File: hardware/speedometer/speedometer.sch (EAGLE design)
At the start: 129 parts, among them IC1 PIC32MX274F256DT-I_PT, IC10 TPS63001DRCT, IC11 TPS63002DRCT, IC12 SN65220DBVRG4, IC2 CSTCE8M00G55-R0, IC3 HM-11, IC4 BQ27441DRZR-G1A, IC5 BQ24075RGTT, IC6 NRF24L01P-T, IC7 CSTCE16M0V53-R0, IC8 24LC024ST, IC9 MAX16054AZT+T, J1 10104111-0001LF, J2 BAT, J3 CONUFL001-SMD-T, J4 Right_sens, J5 Right, J6 Left_sens, J7 Left, Q1 BC817, Q2 BC817, Q3 BC817, Q4 BC817, U1 SN74AHC1G08DBVR, U2 SN74AHC1G08DBVR, X1 TSW-102-07-G-S, X2 TSW-102-07-G-S

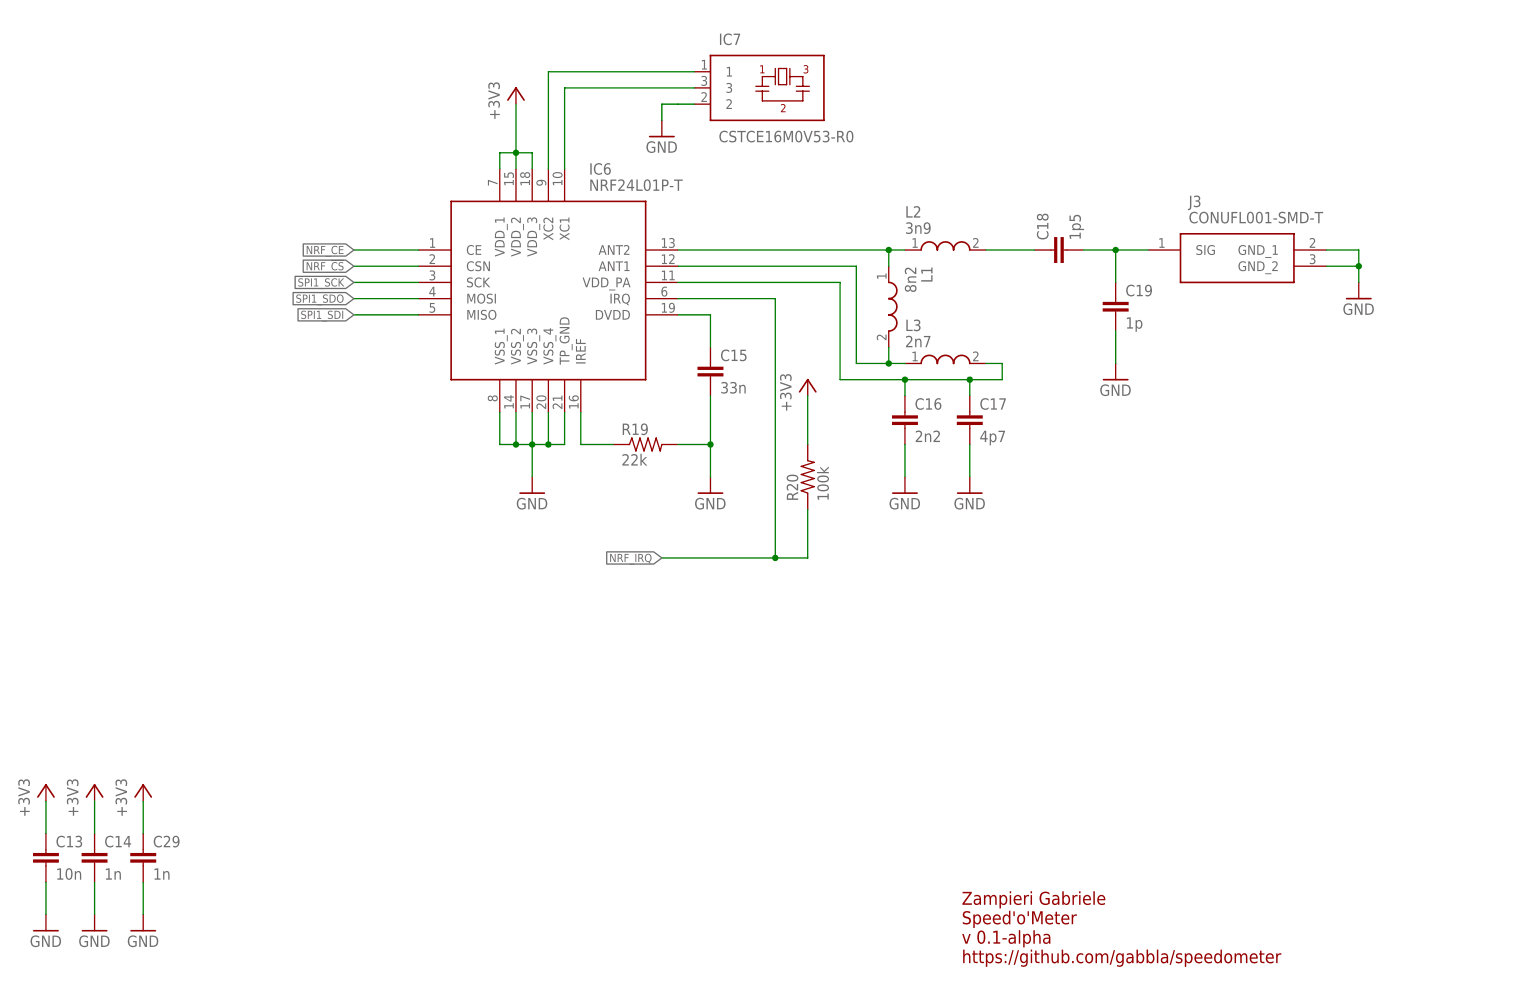
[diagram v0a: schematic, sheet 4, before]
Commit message: wip
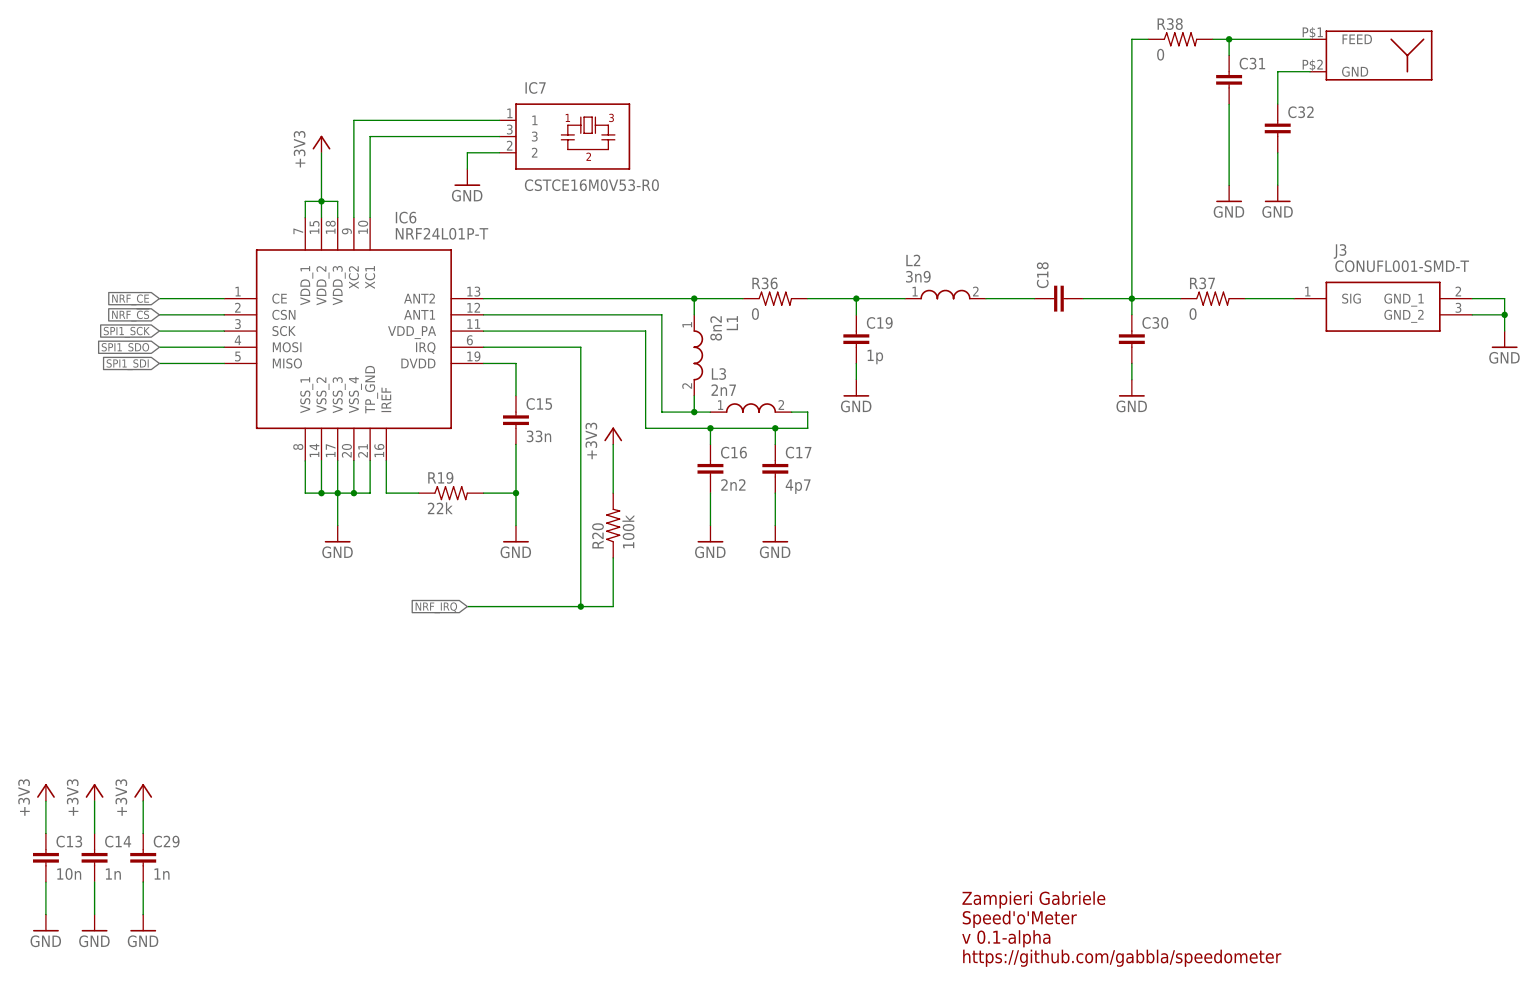
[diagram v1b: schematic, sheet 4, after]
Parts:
- added C30, C31, C32: (no value), rcl:C-EUC0402K
- added R36, R37, R38: 0, rcl:R-US_R0402
- added U$1: M310210, m310210:M310210
- C18: value 1p5 -> (none)
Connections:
- new net N$17: C19.1, L2.P$1, R36.2
- new net N$20: C18.2, C30.1, R37.1, R38.1
- new net N$23: J3.SIG, R37.2
- new net N$36: C32.1, U$1.GND
- net GND: now also C30.2, C31.2, C32.2
- net N$32: now also R36.1; no longer L2.P$1
- net N$37: now also C31.1, R38.2, U$1.FEED; no longer C18.2, C19.1, J3.SIG
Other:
- moved on the sheet: C15, C16, C17, C18, C19, IC6, IC7, J3, L1, L2, L3, R19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
